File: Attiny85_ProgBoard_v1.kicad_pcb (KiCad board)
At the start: 2 copper layers, 1 part, among them U1 ATtiny85V-10PU

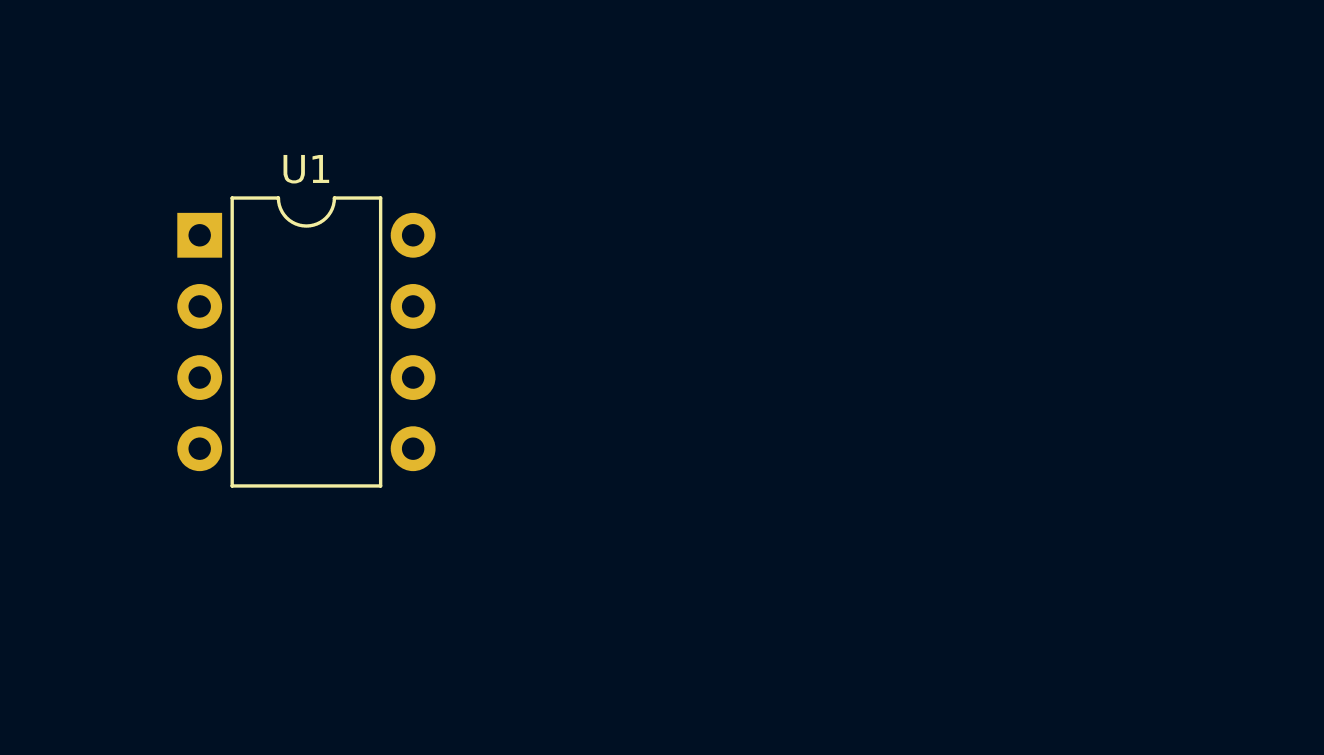
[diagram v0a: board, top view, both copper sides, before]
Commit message: worked on PCB design
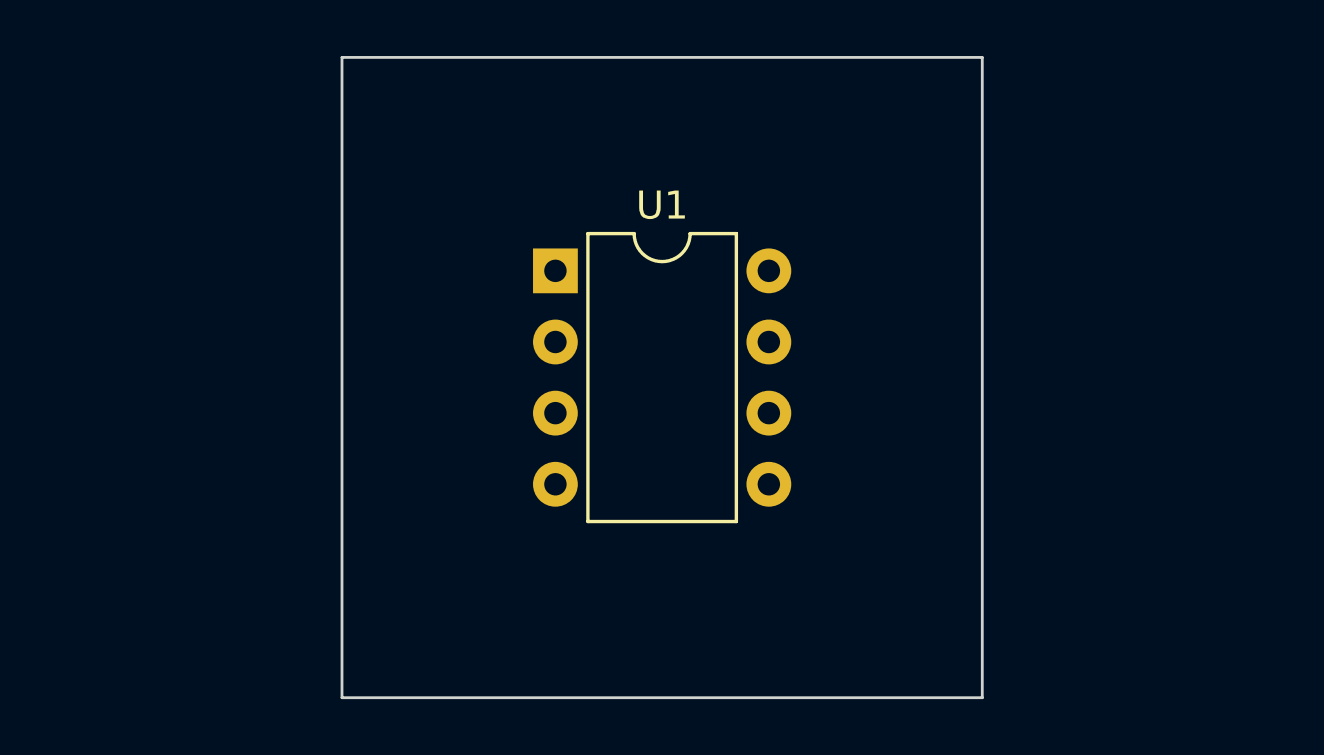
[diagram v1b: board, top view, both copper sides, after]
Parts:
- moved U1 12.8 mm to (139.7, 86.4)
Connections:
- U1 pad 1: Net-(U1-Pad1) -> unconnected-(U1-~{RESET}/PB5-Pad1)
- U1 pad 2: Net-(U1-Pad2) -> unconnected-(U1-XTAL1/PB3-Pad2)
- U1 pad 3: Net-(U1-Pad3) -> unconnected-(U1-XTAL2/PB4-Pad3)
- U1 pad 4: Net-(U1-Pad4) -> unconnected-(U1-GND-Pad4)
- U1 pad 5: Net-(U1-Pad5) -> unconnected-(U1-AREF/PB0-Pad5)
- U1 pad 6: Net-(U1-Pad6) -> unconnected-(U1-PB1-Pad6)
- U1 pad 7: Net-(U1-Pad7) -> unconnected-(U1-PB2-Pad7)
- U1 pad 8: Net-(U1-Pad8) -> unconnected-(U1-VCC-Pad8)
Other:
- board outline added: 22.9 x 22.9 mm
- net class Default removed

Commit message: Designed PCB
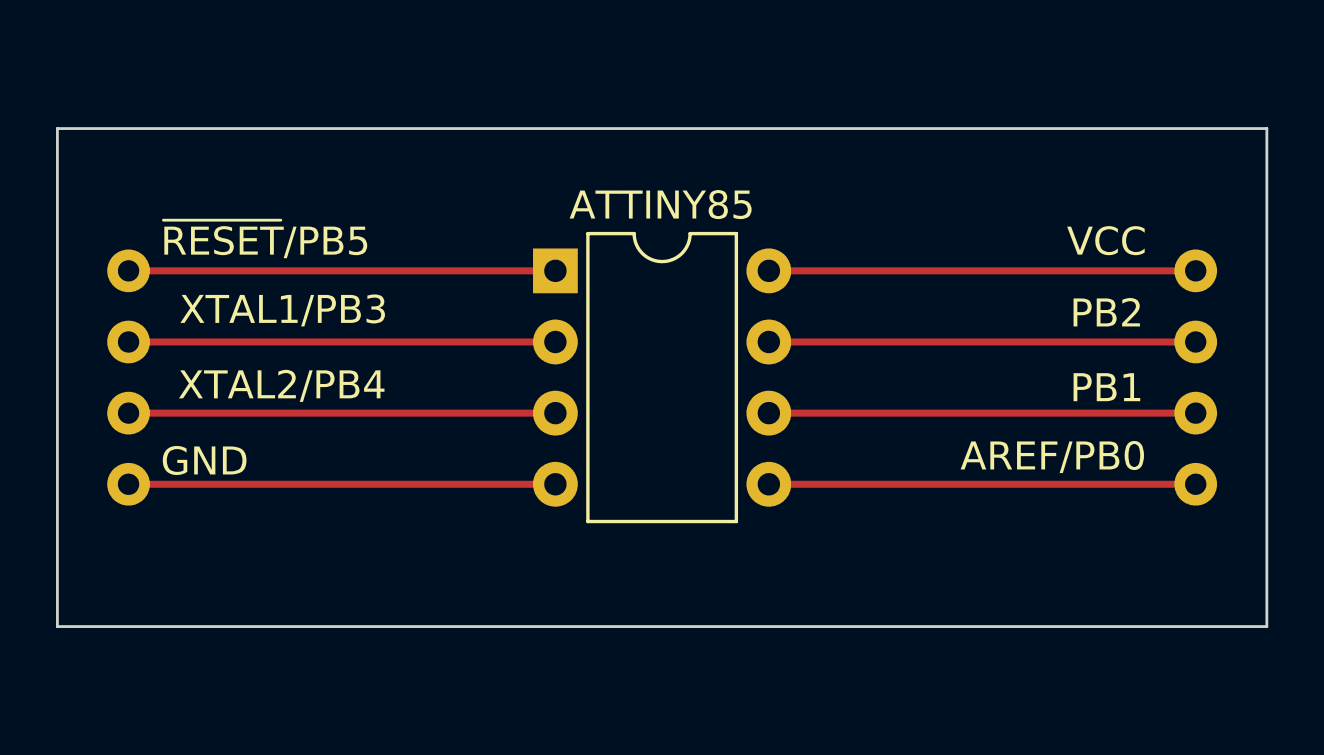
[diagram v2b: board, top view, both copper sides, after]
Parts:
- added AREF/PB0: Conn_01x01_Female, Connector_Pin:PinHole_01x01, F.Cu at (162.6, 94.0)
- added GND: Conn_01x01_Female, Connector_Pin:PinHole_01x01, F.Cu at (124.5, 94.0)
- added PB1: Conn_01x01_Female, Connector_Pin:PinHole_01x01, F.Cu at (162.6, 91.4)
- added PB2: Conn_01x01_Female, Connector_Pin:PinHole_01x01, F.Cu at (162.6, 88.9)
- added VCC: Conn_01x01_Female, Connector_Pin:PinHole_01x01, F.Cu at (162.6, 86.4)
- added XTAL1/PB3: Conn_01x01_Female, Connector_Pin:PinHole_01x01, F.Cu at (124.5, 88.9)
- added XTAL2/PB4: Conn_01x01_Female, Connector_Pin:PinHole_01x01, F.Cu at (124.5, 91.4)
- added ~{RESET}/PB5: Conn_01x01_Female, Connector_Pin:PinHole_01x01, F.Cu at (124.5, 86.4)
- renumbered U1 to ATTINY85
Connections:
- ATTINY85 pad 1: unconnected-(U1-~{RESET}/PB5-Pad1) -> Net-(J7-Pin_1)
- ATTINY85 pad 2: unconnected-(U1-XTAL1/PB3-Pad2) -> Net-(J5-Pin_1)
- ATTINY85 pad 3: unconnected-(U1-XTAL2/PB4-Pad3) -> Net-(J6-Pin_1)
- ATTINY85 pad 4: unconnected-(U1-GND-Pad4) -> Net-(J8-Pin_1)
- ATTINY85 pad 5: unconnected-(U1-AREF/PB0-Pad5) -> Net-(J2-Pin_1)
- ATTINY85 pad 6: unconnected-(U1-PB1-Pad6) -> Net-(J3-Pin_1)
- ATTINY85 pad 7: unconnected-(U1-PB2-Pad7) -> Net-(J4-Pin_1)
- ATTINY85 pad 8: unconnected-(U1-VCC-Pad8) -> Net-(J1-Pin_1)
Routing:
- net Net-(J4-Pin_1): track 0.00 -> 15.2 mm
- net Net-(J3-Pin_1): track 0.00 -> 15.2 mm
- net Net-(J2-Pin_1): track 0.00 -> 15.2 mm
- net Net-(J1-Pin_1): track 0.00 -> 15.2 mm
- net Net-(J8-Pin_1): track 0.00 -> 15.2 mm
- net Net-(J7-Pin_1): track 0.00 -> 15.2 mm
- net Net-(J6-Pin_1): track 0.00 -> 15.2 mm
- net Net-(J5-Pin_1): track 0.00 -> 15.2 mm
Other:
- board size 22.9 x 22.9 mm -> 43.2 x 17.8 mm
